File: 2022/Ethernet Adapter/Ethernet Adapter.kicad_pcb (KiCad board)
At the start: 2 copper layers, 7 parts, among them J1 Conn_01x08, J2 Conn_01x08

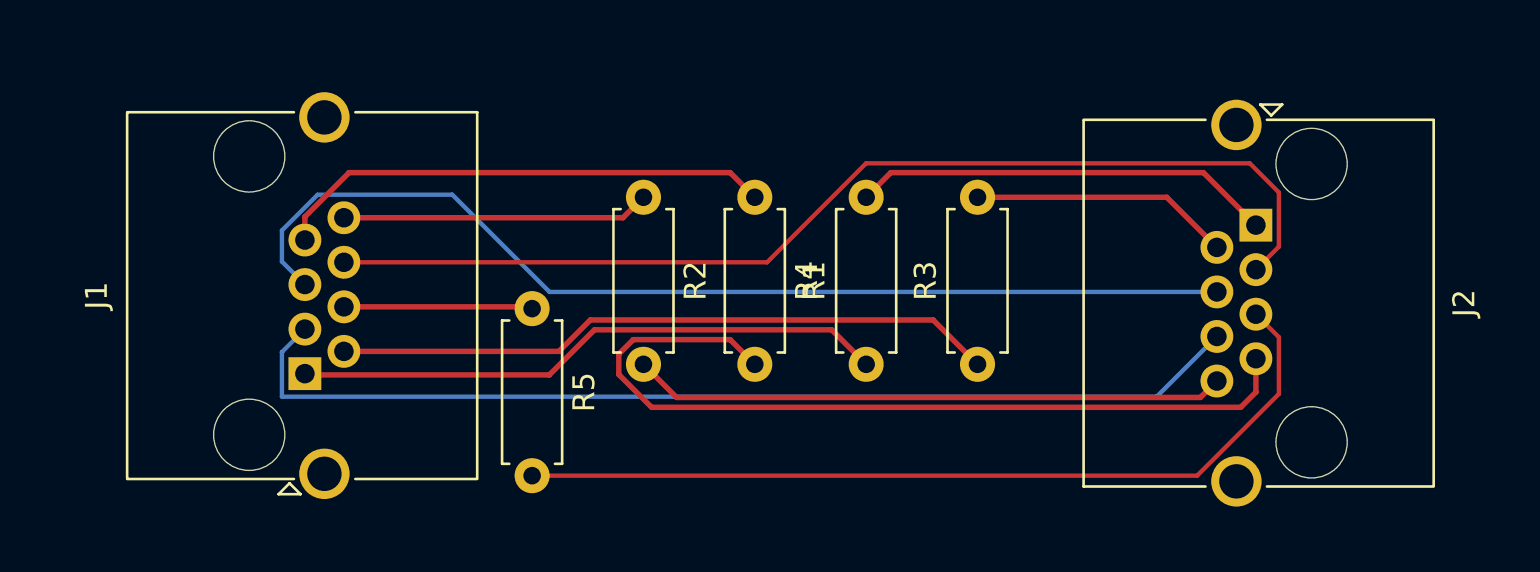
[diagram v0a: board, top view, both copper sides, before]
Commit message: Made changes to board layout
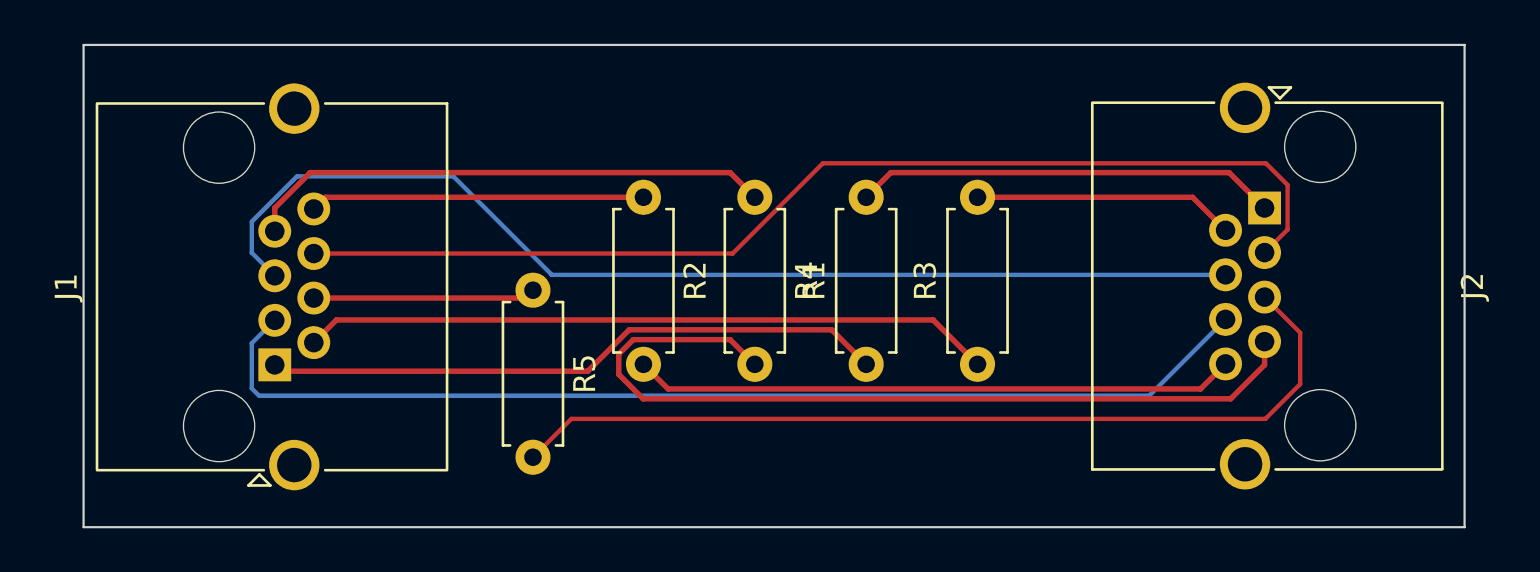
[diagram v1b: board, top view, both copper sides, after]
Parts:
- moved J1 1.43 mm to (87.4, 114.6)
- moved J2 0.87 mm to (132.6, 107.4)
- moved R5 0.84 mm to (99.2, 111.2)
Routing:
- net /TX+: track 47.3 -> 49.5 mm
- net /RX+: track 48.1 -> 50.0 mm
- net Net-(J1-Pad4): track 8.62 -> 10.1 mm
- net Net-(R1-Pad1): track 27.1 -> 28.5 mm
- net /RX-: track 39.7 -> 41.0 mm
- net Net-(J1-Pad8): track 14.1 -> 15.3 mm
- net Net-(J1-Pad7): track 22.9 -> 24.1 mm
- net Net-(J1-Pad2): track 30.3 -> 31.5 mm
- net /TX-: track 49.0 -> 50.1 mm
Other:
- board outline added: 63 x 22 mm
